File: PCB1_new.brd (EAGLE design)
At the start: 101.3 x 47.5 mm, 79 parts

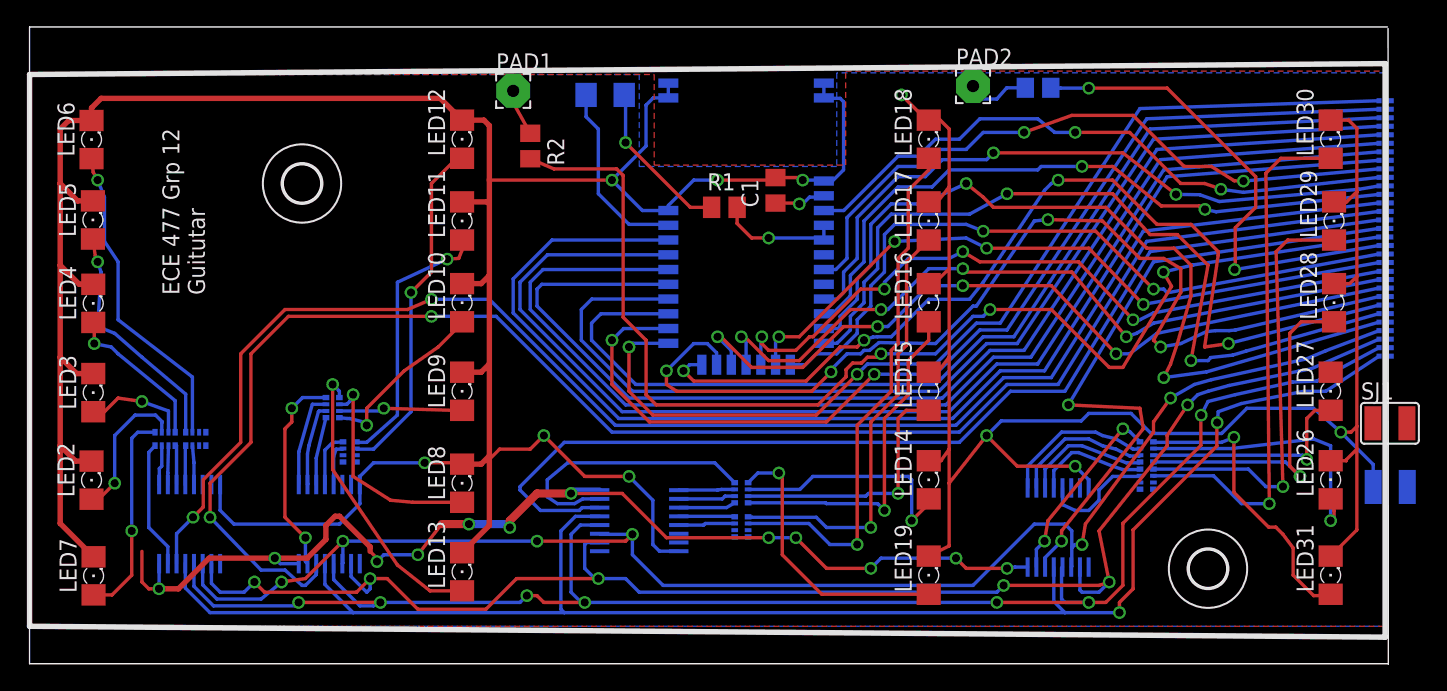
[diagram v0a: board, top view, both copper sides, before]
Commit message: Finished PCB4. Finished gerbers for PCB1, 2, 3, and 4
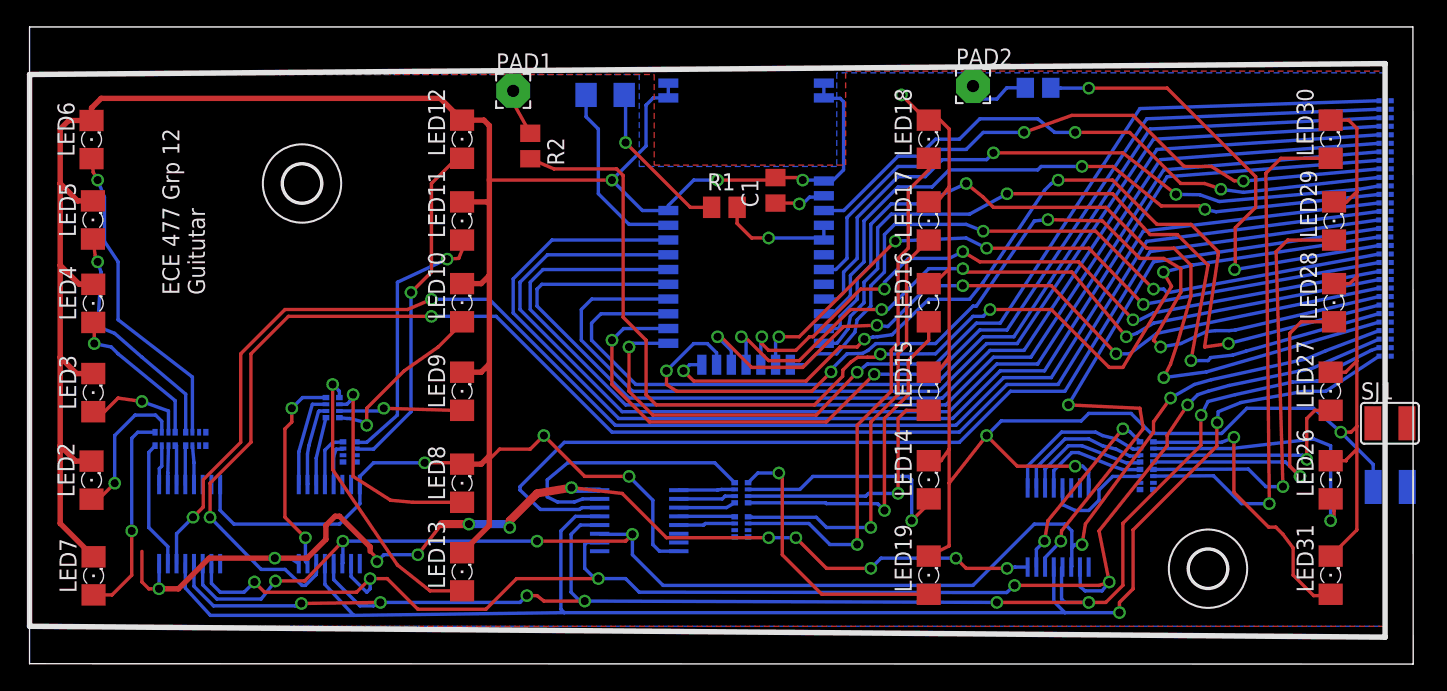
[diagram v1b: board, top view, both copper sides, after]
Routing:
- net GND: track 348.9 -> 352.1 mm
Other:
- board size 101.3 x 47.5 mm -> 103.2 x 47.5 mm
